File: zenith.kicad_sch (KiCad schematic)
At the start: 0 parts

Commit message: wired more of the schematic, added some more parts
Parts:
- added C1, C24, C25, C26: 1uF, symbol Device:C
- added C10, C11, C2, C27, C4, C6, C7, C9: 10uF, symbol Device:C
- added C12, C13, C14, C17, C18: 22uF, symbol Device:C
- added C15: 0.1uF, symbol Device:C
- added C16, C23: 2.2uF, symbol Device:C
- added C19, C20, C21, C22, C28, C29, C30, C31, C32, C8: 100nF, symbol Device:C
- added C3: 44uF, symbol Device:C
- added C5: 47uF, symbol Device:C
- added Card1: TF-01A, lcsc:TF-SMD_TF-01A, symbol lcsc:TF-01A
- added D1: LED, symbol Device:LED
- added FB1: FerriteBead, symbol Device:FerriteBead
- added J1: Screw_Terminal_01x02, symbol Connector:Screw_Terminal_01x02
- added L1, L2: 1uH, symbol Device:L
- added L3: 5.6uH, symbol Device:L
- added R1, R2: 5.1 K, symbol Device:R
- added R10, R12, R13, R16, R17, R18, R19, R20, R21, R3, R4, R5, R6, R8: 10K, symbol Device:R
- added R11: 5.23K, symbol Device:R
- added R14: 100k, symbol Device:R
- added R15: 22.1k, symbol Device:R
- added R7: 383, symbol Device:R
- added R9: 30.1K, symbol Device:R
- added U1: TPS63070RNMR, lcsc:VQFN-HR-15_L3.0-W2.5-P0.50-BL_TPS63070RNMR, symbol lcsc:TPS63070RNMR
- added U2: BMP580, lcsc:LGA-10_L2.0-W2.0-P0.50-TL_BMP580, symbol lcsc:BMP580
- added U3: BQ25883RGER, lcsc:VFQFPN-24_L4.0-W4.0-P0.50-BL-EP2.8, symbol lcsc:BQ25883RGER
- added U4: ICM-45686, lcsc:LGA-14_L3.0-W2.5-P0.50-TL, symbol lcsc:ICM-45686
- added U5: STM32F722RETx, Package_QFP:LQFP-64_10x10mm_P0.5mm, symbol MCU_ST_STM32F7:STM32F722RETx
- added U6: LMR51430, Package_TO_SOT_SMD:SOT-23-6, symbol Regulator_Switching:LMR51430
- added USB1: TYPE-C 16PIN 2MD(073), lcsc:USB-C-SMD_TYPE-C-6PIN-2MD-073, symbol lcsc:TYPE-C16PIN2MD(073)
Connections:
- new net: R14.2, R15.1, U6.4 (FB)
- new net: R1.2, USB1.4 (CC1)
- new net: C8.1, U1.3 (Vaux)
- new net: R12.1, U1.1 (PS/SYNC), U1.14 (EN)
- new net: L2.2, U1.11 (L1)
- new net: R13.1, U1.2 (PG)
- new net: R13.2, U1.5 (FB)
- new net: L2.1, U1.9 (L2)
- new net: C2.1, L1.1, U3.21 (PMID), U3.22 (PMID)
- new net: R2.2, USB1.10 (CC2)
- new net: C23.1, U5.30 (VCAP_1)
- new net: R10.1, R11.2, R9.1, U3.7 (TS)
- new net: FB1.2, U5.13 (VDDA)
- new net: R7.1, U3.8 (ILIM)
- new net: C15.2, L3.1, U6.2 (SW)
- new net: C5.1, U3.12 (BTST)
- new net: D1.2 (A), U3.2 (STAT)
- new net: C15.1, U6.6 (CB)
- new net: D1.1 (K), R3.1
- new net +3.3V: C17.1, C18.1, C19.1, C20.1, C21.1, C22.1, C24.1, C25.1, C26.1, C27.1, C28.1, C29.1, C30.1, C31.1, C32.1, Card1.4 (VDD), FB1.1, L3.2, R14.1, R16.1, R17.1, R18.1, R19.1, R20.1, R21.1, R3.2, R4.1, R5.1, R6.1, R8.2, U2.1 (VDDIO), U2.10 (VDD), U4.5 (VDDIO), U4.8 (VDD), U5.1 (VBAT), U5.19 (VDD), U5.32 (VDD), U5.48 (VDD), U5.64 (VDD)
- new net +5V: C12.1, C13.1, C14.1, C9.1, U1.7 (Vout), U1.8 (Vout)
- new net +BAT: C4.1, J1.1 (Pin_1), U3.13 (BAT)
- new net BAT-: C1.1, J1.2 (Pin_2)
- new net BMP_INT: U2.7 (INT)
- new net BMP_SCK: U2.2 (SCK)
- new net BMP_SDI: U2.4 (SDI)
- new net BQ_CE: U3.3 (~{CE})
- new net BQ_INT: R4.2, U3.6 (~{INT})
- new net BQ_PG: R8.1, U3.9 (~{PG})
- new net BQ_SCL: R5.2, U3.5 (SCL)
- new net BQ_SDA: R6.2, U3.4 (SDA)
- new net BTST: C5.2, L1.2, U3.17 (SW), U3.18 (SW)
- new net GND: C10.2, C11.2, C12.2, C13.2, C14.2, C16.2, C17.2, C18.2, C19.2, C2.2, C20.2, C21.2, C22.2, C23.2, C24.2, C25.2, C26.2, C27.2, C28.2, C29.2, C3.2, C30.2, C31.2, C32.2, C4.2, C6.1, C7.2, C8.2, C9.2, Card1.10 (GND), Card1.11 (GND), Card1.12 (GND), Card1.13 (GND), Card1.6 (VSS), R1.1, R10.2, R15.2, R2.1, R7.2, R9.2, U1.10 (PGND), U1.15 (Vsel), U1.4 (GND), U1.6 (FB2), U2.3 (VSS), U2.5 (SDO), U2.6 (CSB), U2.8 (VSS), U2.9 (VSS), U3.19 (GND), U3.20 (GND), U4.6 (GND), U5.12 (VSSA), U5.18 (VSS), U5.31 (VSS), U5.47 (VSS), U5.63 (VSS), U6.1 (GND), USB1.1 (GND), USB1.12 (GND), USB1.13 (SHELL), USB1.14 (SHELL)
- new net ICM_CS: U4.12 (AP_CS)
- new net ICM_INT1: U4.4 (INT1/INT)
- new net ICM_INT2: U4.9 (INT2/FSYNC/CLKIN)
- new net ICM_SCK: U4.13 (AP_SCL/AP_SCLK)
- new net ICM_SDI: U4.14 (AP_SDA/AP_SDIO/AP_SDI)
- new net ICM_SDO: U4.1 (AP_SDO/AP_AD0)
- new net SD_CD: Card1.9 (CD)
- new net SD_CLK: Card1.5 (CLK(SCLK)), R16.2
- new net SD_CMD: Card1.3 (CMD(DI)), R17.2
- new net SD_DAT0: Card1.7 (DAT0(D0)), R21.2
- new net SD_DAT1: Card1.8 (DAT1(RSV)), R20.2
- new net SD_DAT2: Card1.1 (DAT2(RSV)), R19.2
- new net SD_DAT3: Card1.2 (CDDAT3(CS)), R18.2
- new net USB_DN: USB1.5 (DN2), USB1.7 (DN1)
- new net USB_DP: USB1.6 (DP1), USB1.8 (DP2)
- new net VBUS: C1.2, U3.23 (VBUS), USB1.11 (VBUS), USB1.2 (VBUS)
- new net VREGN: C6.2, R11.1, U3.11 (REGN)
- new net VSYS: C10.1, C11.1, C16.1, C3.1, C7.1, R12.2, U1.12 (Vin), U1.13 (Vin), U3.15 (SYS), U3.16 (SYS), U6.3 (VIN), U6.5 (EN)
- no-connect marks 0 -> 11
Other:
- note added: "Battery Charger"

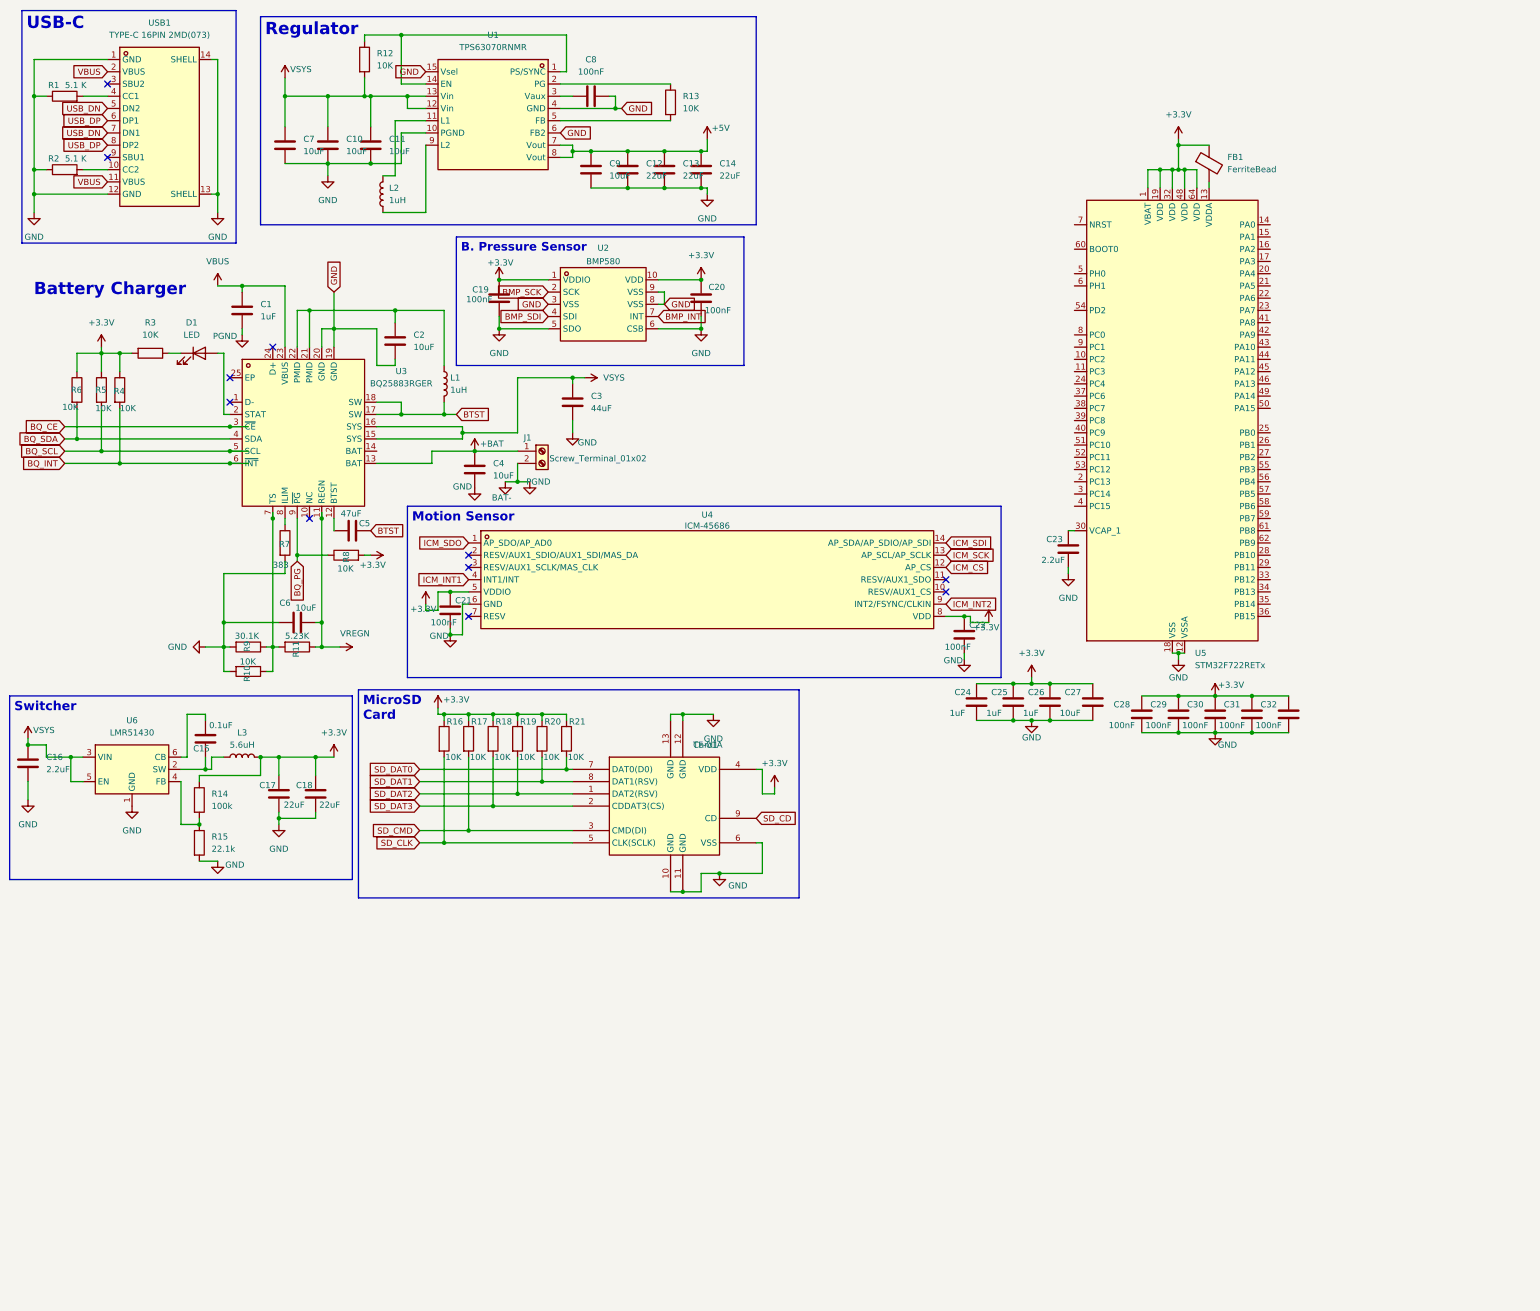
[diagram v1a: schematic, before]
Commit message: organization, more wires!
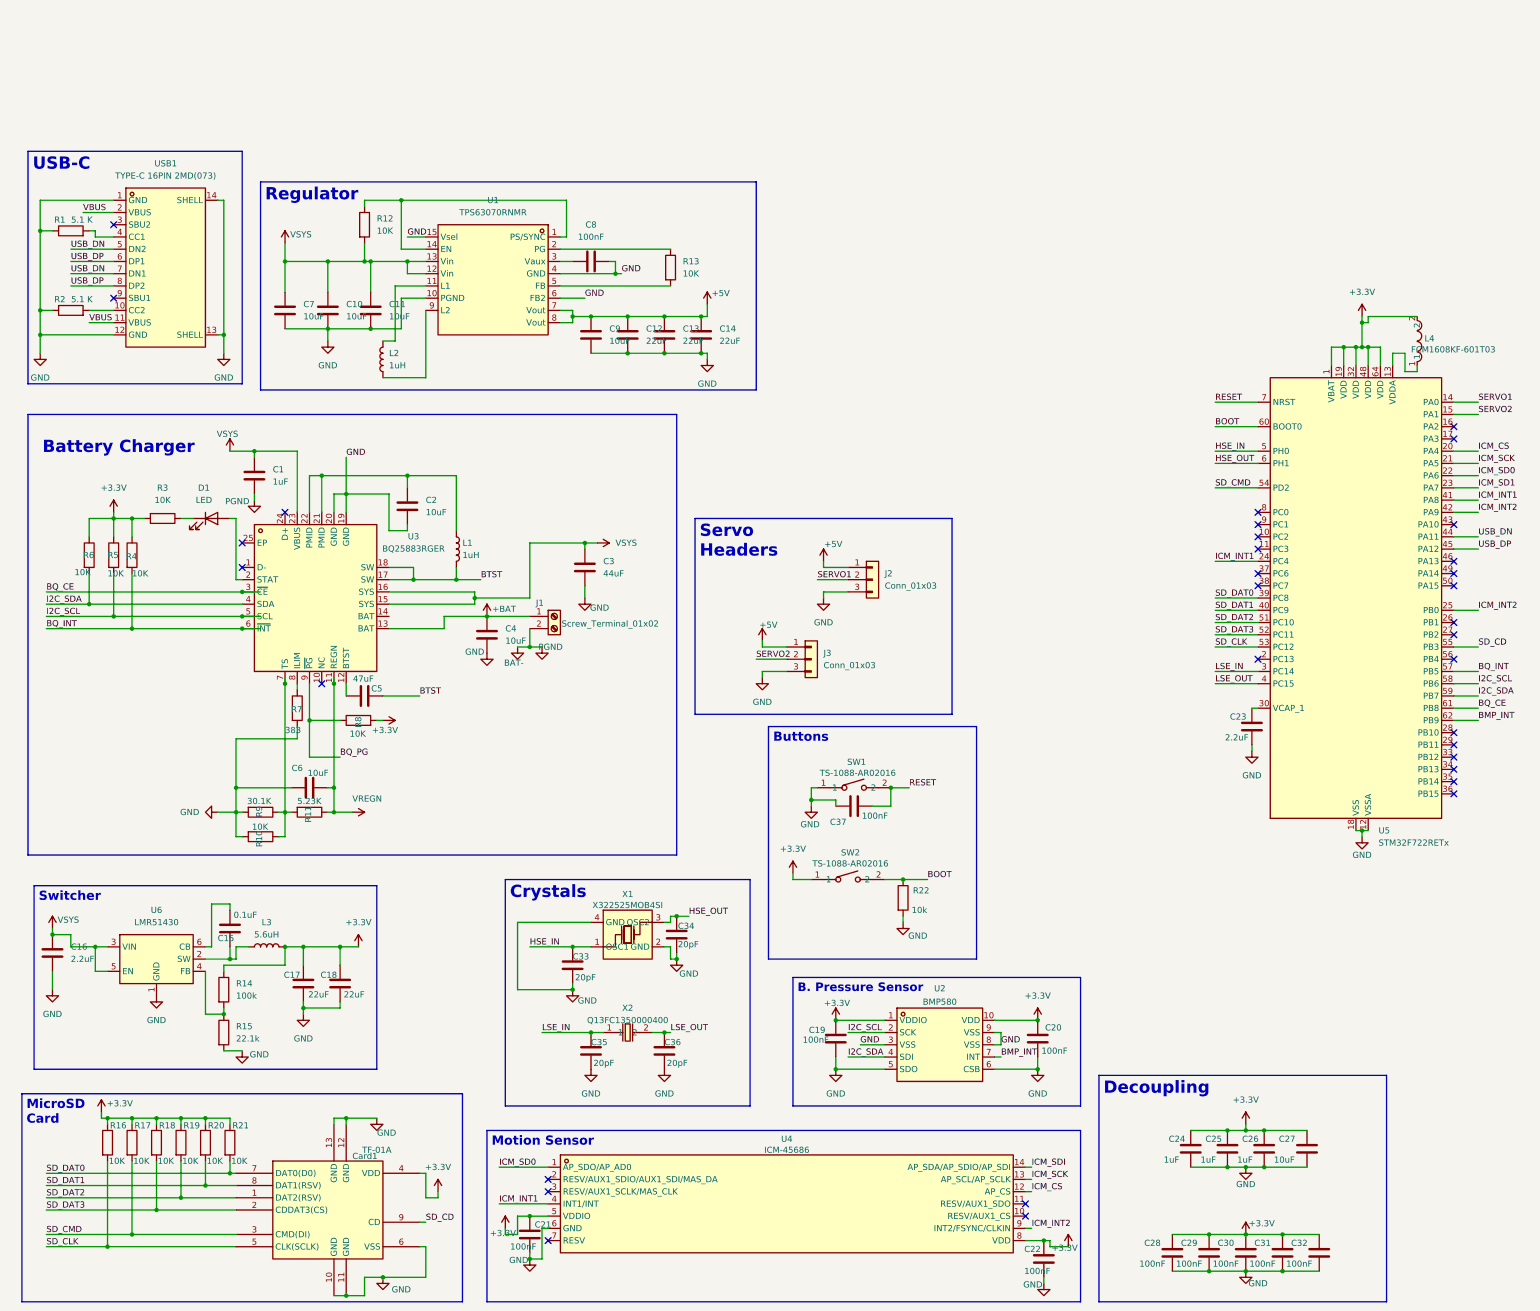
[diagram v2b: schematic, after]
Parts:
- removed FB1: FerriteBead, symbol Device:FerriteBead
- added C33, C34, C35, C36: 20pF, symbol Device:C
- added C37: 100nF, symbol Device:C
- added J2, J3: Conn_01x03, symbol Connector_Generic:Conn_01x03
- added L4: FCM1608KF-601T03, lcsc:L0603, symbol lcsc:FCM1608KF-601T03
- added R22: 10k, symbol Device:R
- added SW1, SW2: TS-1088-AR02016, lcsc:SW-SMD_L3.9-W3.0-P4.45, symbol lcsc:TS-1088-AR02016
- added X1: X322525MOB4SI, lcsc:CRYSTAL-SMD_4P-L3.2-W2.5-BL, symbol lcsc:X322525MOB4SI
- added X2: Q13FC1350000400, lcsc:FC-135R_L3.2-W1.5, symbol lcsc:Q13FC1350000400
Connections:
- net BMP_SCK is gone; now on net I2C_SCL: U2.2 (SCK)
- net BMP_SDI is gone; now on net I2C_SDA: U2.4 (SDI)
- net BQ_SCL is gone; now on net I2C_SCL: R5.2, U3.5 (SCL)
- net BQ_SDA is gone; now on net I2C_SDA: R6.2, U3.4 (SDA)
- net ICM_SDO is gone; now on net ICM_SD0: U4.1 (AP_SDO/AP_AD0)
- net +3.3V: now also L4.2, SW2.1
- net +5V: now also J2.1 (Pin_1), J3.1 (Pin_1)
- net BMP_INT: now also U5.62 (PB9)
- net BQ_CE: now also U5.61 (PB8)
- net BQ_INT: now also U5.57 (PB5)
- net GND: now also C33.2, C34.2, C35.2, C36.2, C37.1, J2.3 (Pin_3), J3.3 (Pin_3), R22.2, SW1.1, X1.2 (GND), X1.4 (GND)
- net ICM_CS: now also U5.20 (PA4)
- net ICM_INT1: now also U5.24 (PC4), U5.41 (PA8)
- net ICM_INT2: now also U5.25 (PB0), U5.42 (PA9)
- net ICM_SCK: now also U5.21 (PA5)
- net SD_CD: now also U5.55 (PB3)
- net SD_CLK: now also U5.53 (PC12)
- net SD_CMD: now also U5.54 (PD2)
- net SD_DAT0: now also U5.39 (PC8)
- net SD_DAT1: now also U5.40 (PC9)
- net SD_DAT2: now also U5.51 (PC10)
- net SD_DAT3: now also U5.52 (PC11)
- net USB_DN: now also U5.44 (PA11)
- net USB_DP: now also U5.45 (PA12)
- net VBUS: no longer C1.2, U3.23 (VBUS)
- net VSYS: now also C1.2, U3.23 (VBUS)
- net at U5.13 (VDDA): now also L4.1
- net SERVO1: now reaches U5.14 (PA0)
- net SERVO1: now also J2.2 (Pin_2)
- net SERVO2: now reaches U5.15 (PA1)
- net SERVO2: now also J3.2 (Pin_2)
- net ICM_SD0: now reaches U5.22 (PA6)
- net ICM_SD1: now reaches U5.23 (PA7)
- net LSE_IN: now reaches U5.3 (PC14)
- net LSE_IN: now also C35.1, X2.1
- net LSE_OUT: now reaches U5.4 (PC15)
- net LSE_OUT: now also C36.1, X2.2
- net HSE_IN: now reaches U5.5 (PH0)
- net HSE_IN: now also C33.1, X1.1 (OSC1)
- net I2C_SCL: now reaches U5.58 (PB6)
- net I2C_SDA: now reaches U5.59 (PB7)
- net HSE_OUT: now reaches U5.6 (PH1)
- net HSE_OUT: now also C34.1, X1.3 (OSC2)
- net BOOT: now reaches U5.60 (BOOT0)
- net BOOT: now also R22.1, SW2.2
- net RESET: now reaches U5.7 (NRST)
- net RESET: now also C37.2, SW1.2
- no-connect marks 11 -> 33
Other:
- moved on the sheet: C1, C10, C11, C12, C13, C14, C15, C16, C17, C18, C19, C2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

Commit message: finished schematic
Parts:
- L2: value 1uH -> 1.5uH
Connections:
- net ICM_SD1 is gone; now on net ICM_SDI: U5.23 (PA7)
- net BMP_INT: now also U5.56 (PB4); no longer U5.62 (PB9)
- net ICM_INT1: now also U5.26 (PB1); no longer U5.24 (PC4)
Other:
- note added: "Power"
- note added: "Sensors + Peripherals"
- moved on the sheet: C1, C10, C11, C12, C13, C14, C15, C16, C17, C18, C19, C2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

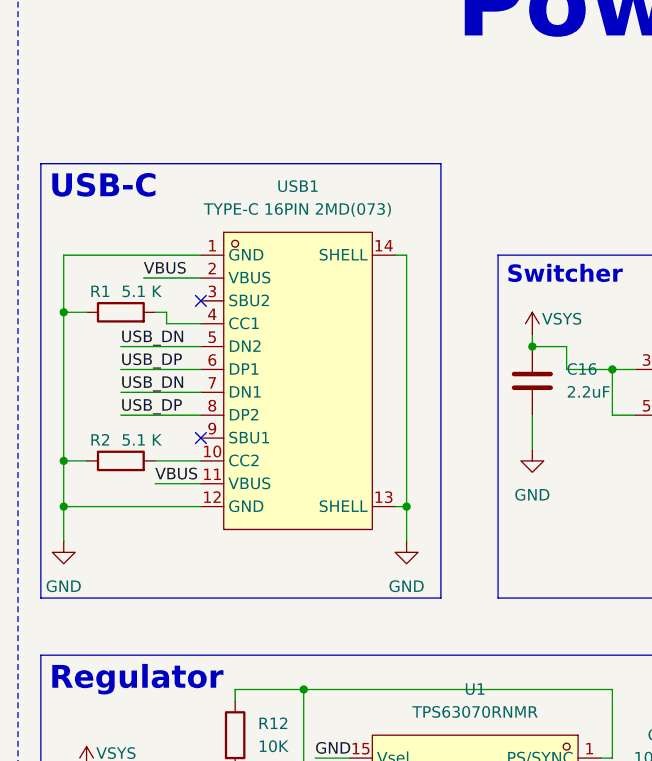
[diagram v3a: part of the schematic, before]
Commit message: placed components, began routing
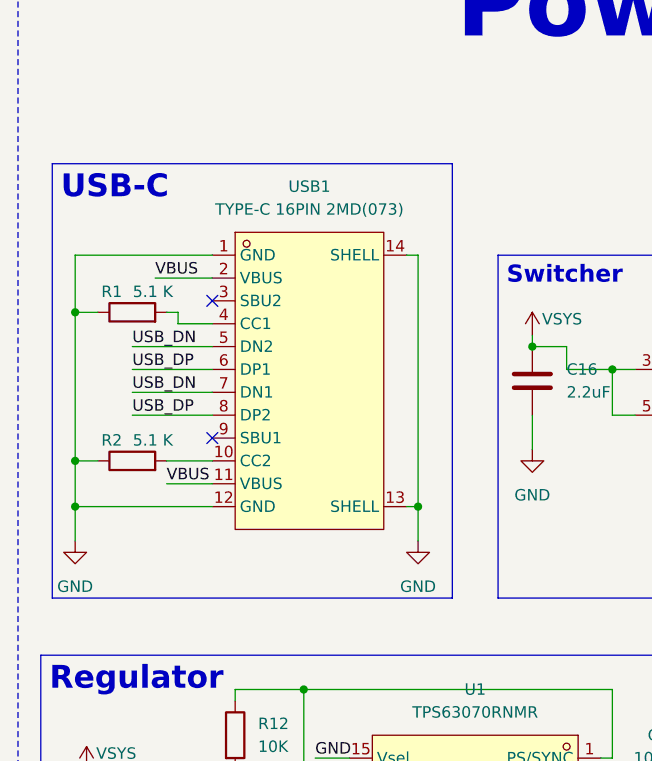
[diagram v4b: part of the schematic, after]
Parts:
- C1, C10, C11, C16, C2, C23, C24, C25, C26, C27, C4, C6, C7, C9: footprint (none) -> Capacitor_SMD:C_0402_1005Metric
- C12, C13, C14, C17, C18, C3, C5: footprint (none) -> Capacitor_SMD:C_0805_2012Metric
- C15, C19, C20, C21, C22, C28, C29, C30, C31, C32, C33, C34, C35, C36, C37, C8: footprint (none) -> Capacitor_SMD:C_0201_0603Metric
- D1: footprint (none) -> LED_SMD:LED_0402_1005Metric
- J1: footprint (none) -> TerminalBlock:TerminalBlock_Xinya_XY308-2.54-2P_1x02_P2.54mm_Horizontal
- J2, J3: footprint (none) -> Connector_PinHeader_2.54mm:PinHeader_1x03_P2.54mm_Vertical
- L1: footprint (none) -> lcsc:L2520
- L2: footprint (none) -> lcsc:IND-SMD_L4.0-W4.0-A
- L3: footprint (none) -> lcsc:IND-SMD_L3.0-W3.0
- R1, R10, R11, R12, R13, R15, R16, R17, R18, R19, R2, R20, R21, R22, R3, R4, R5, R6, R7, R8, R9: footprint (none) -> Resistor_SMD:R_0201_0603Metric
- R14: footprint (none) -> Resistor_SMD:R_0402_1005Metric
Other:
- moved on the sheet: R1, R2, USB1
